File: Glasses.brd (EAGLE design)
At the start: 157.5 x 68.6 mm, 260 parts, among them U1 APA1022020, U10 APA1022020, U100 APA1022020, U101 APA1022020, U102 APA1022020, U103 APA1022020, U104 APA1022020, U105 APA1022020, U106 APA1022020, U107 APA1022020, U108 APA1022020, U109 APA1022020, U11 APA1022020, U110 APA1022020, U111 APA1022020, U112 APA1022020, U113 APA1022020, U114 APA1022020, U115 APA1022020, U116 APA1022020, U117 APA1022020, U118 APA1022020, U119 APA1022020, U12 APA1022020, U120 APA1022020, U121 APA1022020, U122 APA1022020, U123 APA1022020, U124 APA1022020, U125 APA1022020, U126 APA1022020, U127 APA1022020, U128 APA1022020, U129 APA1022020, U13 APA1022020, U130 APA1022020, U131 APA1022020, U132 APA1022020, U133 APA1022020, U134 APA1022020, U135 APA1022020, U136 APA1022020, U137 APA1022020, U138 APA1022020, U139 APA1022020, U14 APA1022020, U140 APA1022020, U141 APA1022020, U142 APA1022020, U143 APA1022020, U144 APA1022020, U145 APA1022020, U146 APA1022020, U147 APA1022020, U148 APA1022020, U149 APA1022020, U15 APA1022020, U150 APA1022020, U151 APA1022020, U152 APA1022020, U153 APA1022020, U154 APA1022020, U155 APA1022020, U156 APA1022020, U157 APA1022020, U158 APA1022020, U159 APA1022020, U16 APA1022020, U160 APA1022020, U161 APA1022020, U162 APA1022020, U163 APA1022020, U164 APA1022020, U165 APA1022020, U166 APA1022020, U167 APA1022020, U168 APA1022020, U169 APA1022020, U17 APA1022020, U170 APA1022020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

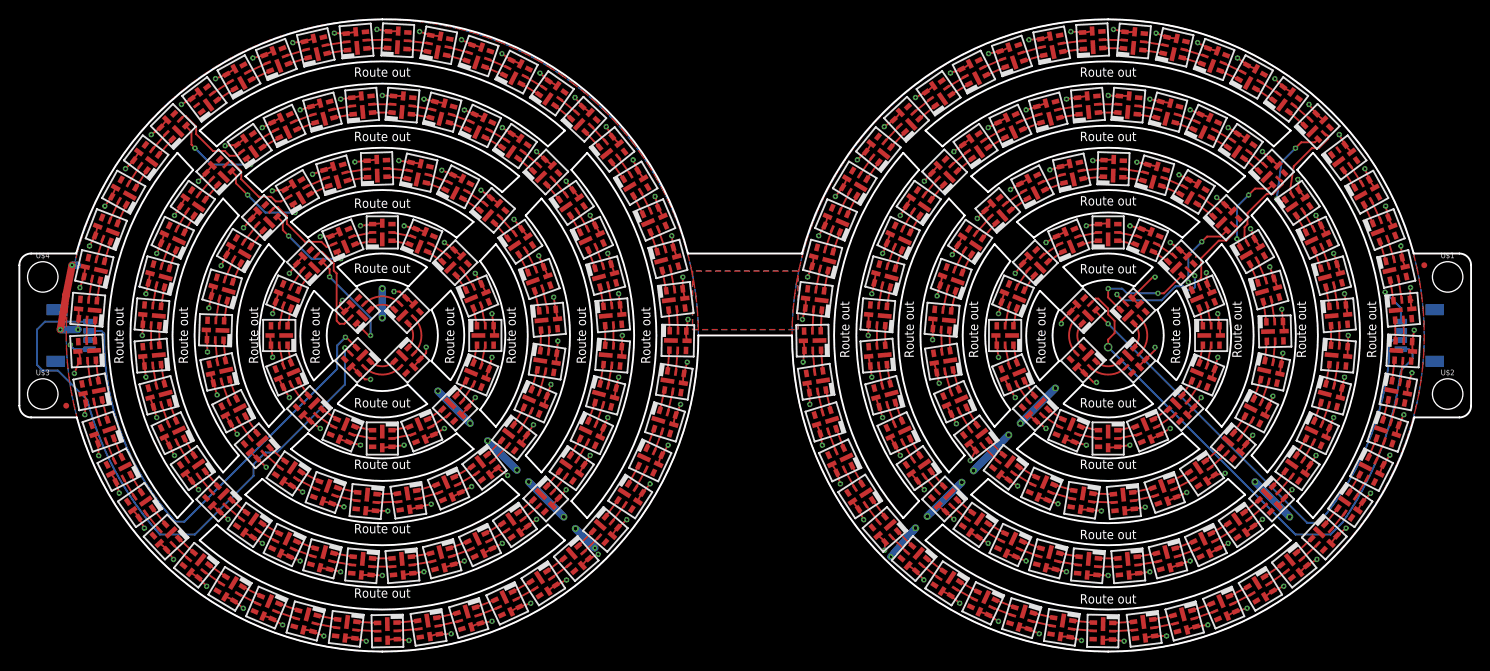
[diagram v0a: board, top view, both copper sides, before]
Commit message: glasses brd
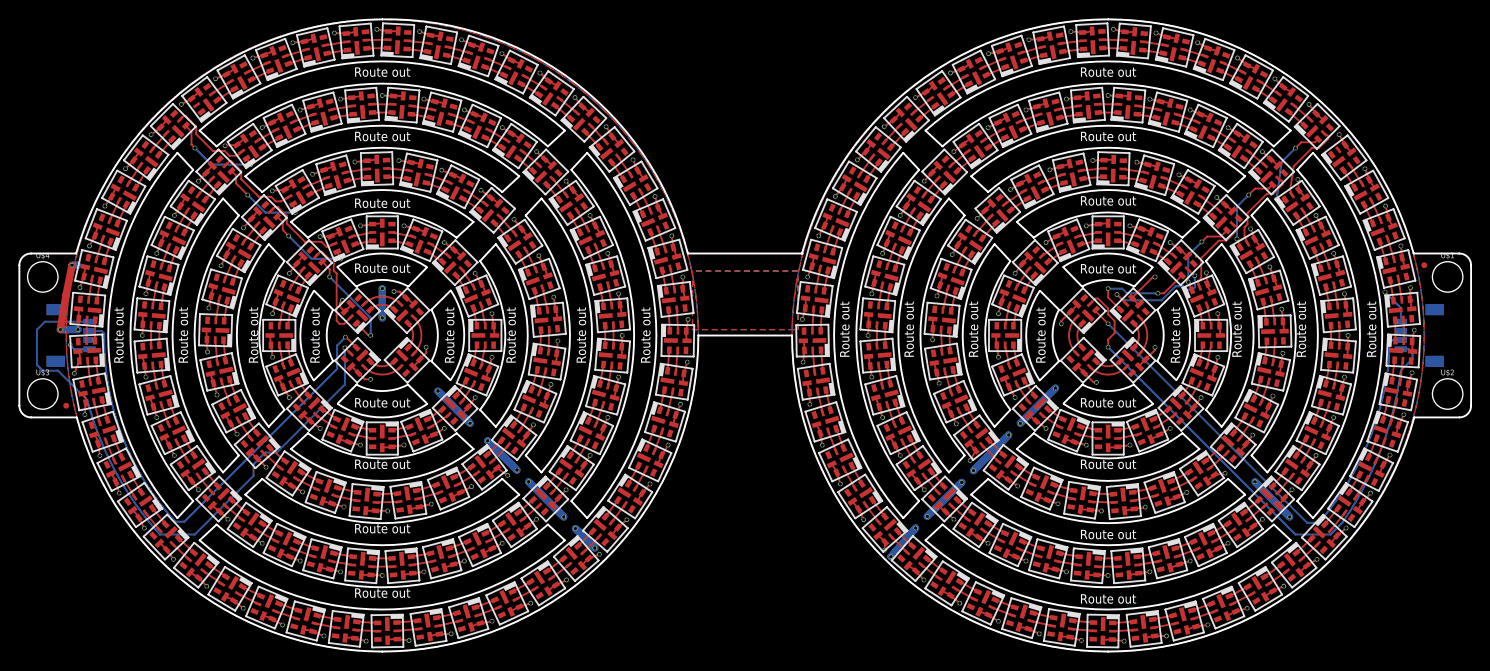
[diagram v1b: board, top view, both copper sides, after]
